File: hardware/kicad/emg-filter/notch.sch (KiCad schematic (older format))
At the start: 9 parts, among them U1 LM4565

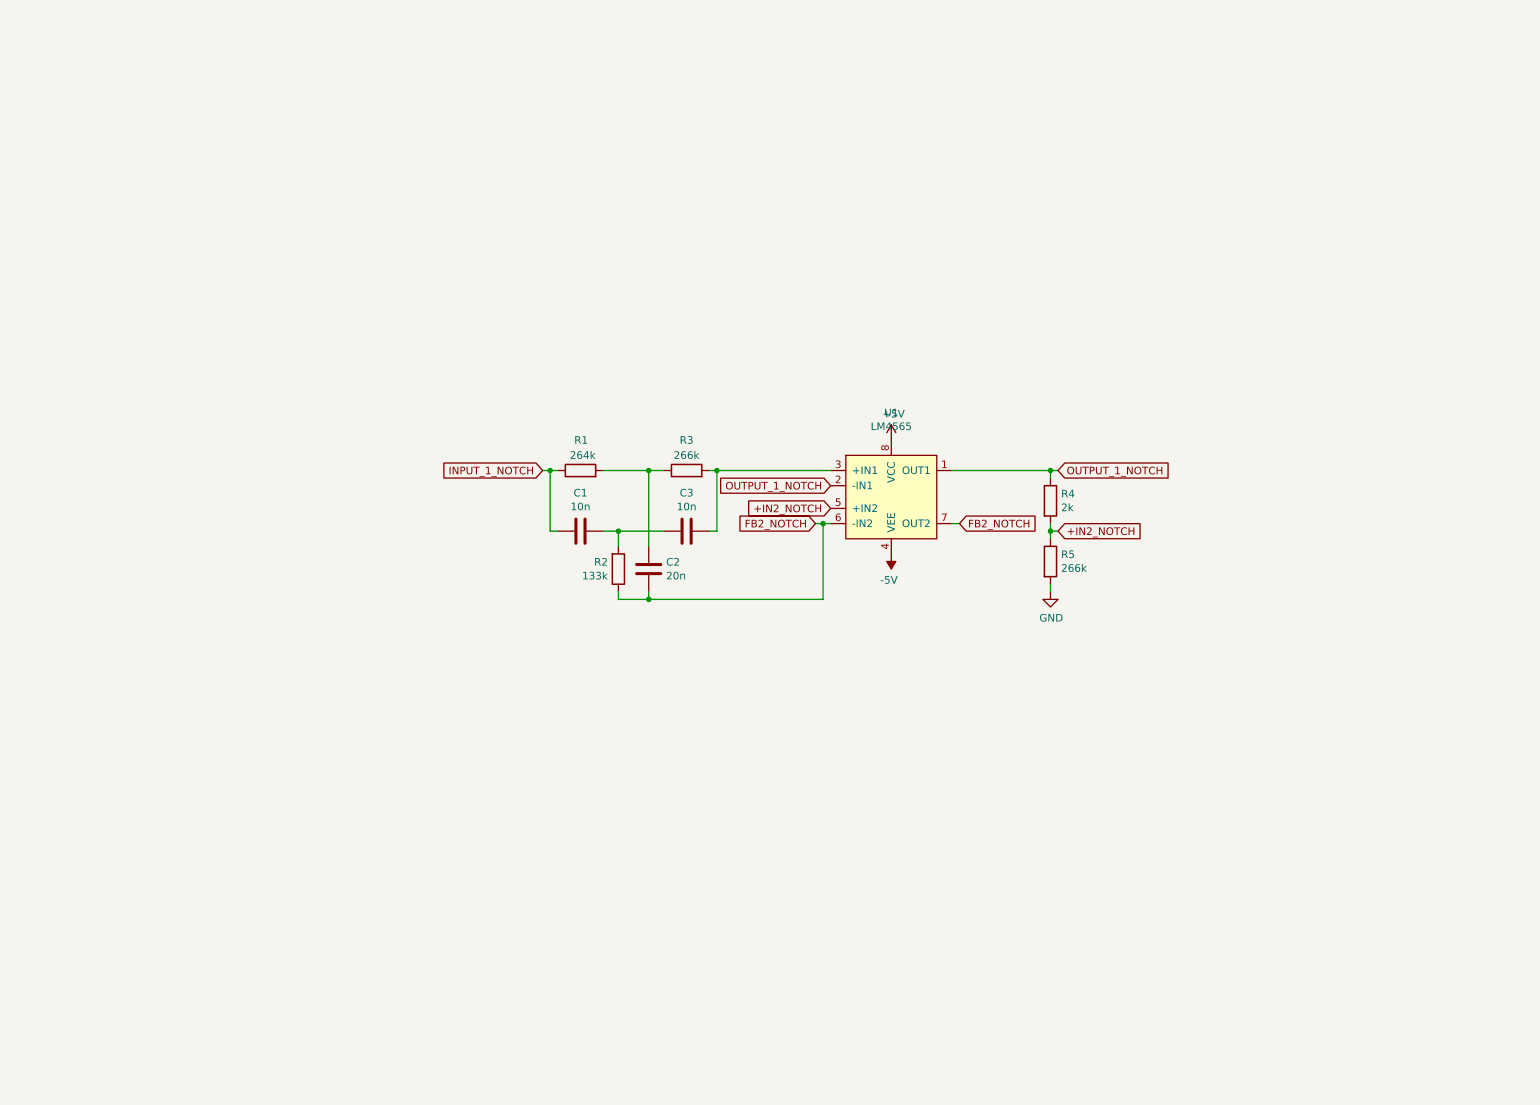
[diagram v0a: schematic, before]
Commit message: notch x16
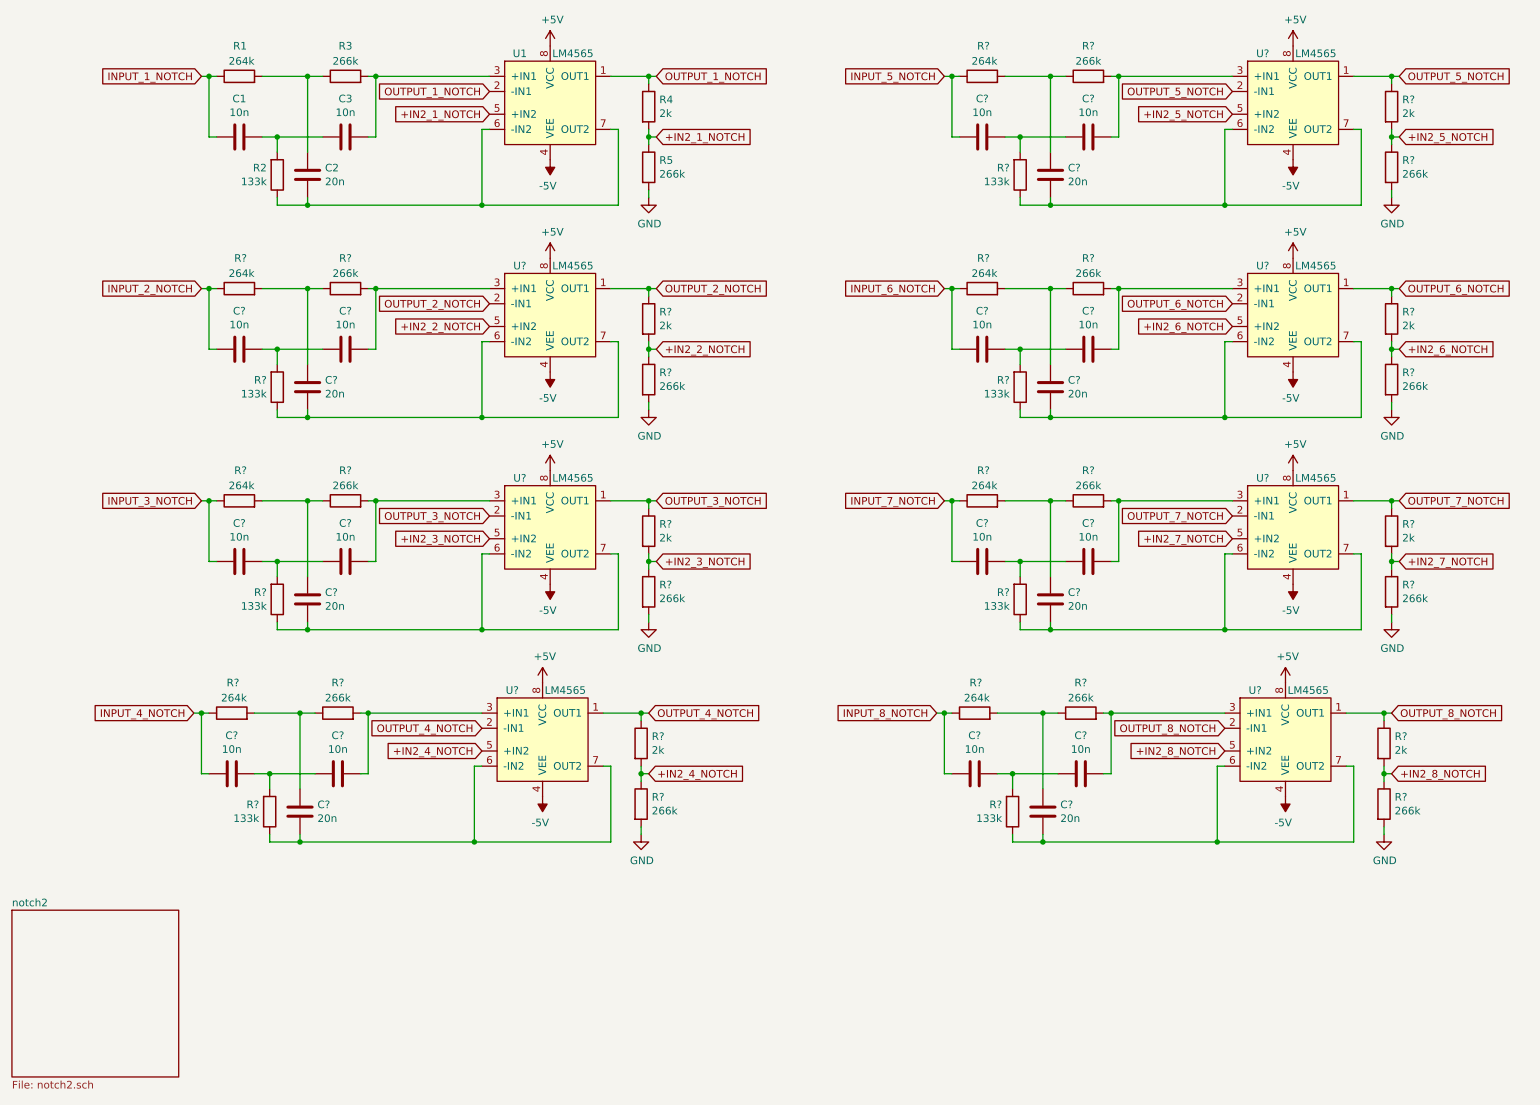
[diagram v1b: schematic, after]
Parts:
- added C? (x7): 20n, symbol Device:C
- added C? (x14): 10n, symbol Device:C
- added R? (x14): 266k, symbol Device:R
- added R? (x7): 133k, symbol Device:R
- added R? (x7): 2k, symbol Device:R
- added R? (x7): 264k, symbol Device:R
- added U? (x7): LM4565, symbol emg-filter:LM4565
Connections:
- net +5V: now also U?.8 (VCC), U?.8 (VCC), U?.8 (VCC), U?.8 (VCC), U?.8 (VCC), U?.8 (VCC), U?.8 (VCC)
- net -5V: now also U?.4 (VEE), U?.4 (VEE), U?.4 (VEE), U?.4 (VEE), U?.4 (VEE), U?.4 (VEE), U?.4 (VEE)
- net GND: now also R?.2, R?.2, R?.2, R?.2, R?.2, R?.2, R?.2
- net +IN2_NOTCH renamed +IN2_1_NOTCH
- net FB2_NOTCH: no longer names the net of C2.1, R2.1, U1.6 (-IN2), U1.7 (OUT2)
- new net: C?.1, R?.2, U?.3 (+IN1) (x7)
- new net: C?.1, R?.1, U?.6 (-IN2), U?.7 (OUT2) (x7)
- new net: C?.2, R?.1, R?.2 (x7)
- new net: C?.1, C?.2, R?.2 (x7)
- new net +IN2_2_NOTCH: R?.1, R?.2, U?.5 (+IN2)
- new net +IN2_3_NOTCH: R?.1, R?.2, U?.5 (+IN2)
- new net +IN2_4_NOTCH: R?.1, R?.2, U?.5 (+IN2)
- new net +IN2_5_NOTCH: R?.1, R?.2, U?.5 (+IN2)
- new net +IN2_6_NOTCH: R?.1, R?.2, U?.5 (+IN2)
- new net +IN2_7_NOTCH: R?.1, R?.2, U?.5 (+IN2)
- new net +IN2_8_NOTCH: R?.1, R?.2, U?.5 (+IN2)
- new net INPUT_2_NOTCH: C?.2, R?.1
- new net INPUT_3_NOTCH: C?.2, R?.1
- new net INPUT_4_NOTCH: C?.2, R?.1
- new net INPUT_5_NOTCH: C?.2, R?.1
- new net INPUT_6_NOTCH: C?.2, R?.1
- new net INPUT_7_NOTCH: C?.2, R?.1
- new net INPUT_8_NOTCH: C?.2, R?.1
- new net OUTPUT_2_NOTCH: R?.1, U?.1 (OUT1), U?.2 (-IN1)
- new net OUTPUT_3_NOTCH: R?.1, U?.1 (OUT1), U?.2 (-IN1)
- new net OUTPUT_4_NOTCH: R?.1, U?.1 (OUT1), U?.2 (-IN1)
- new net OUTPUT_5_NOTCH: R?.1, U?.1 (OUT1), U?.2 (-IN1)
- new net OUTPUT_6_NOTCH: R?.1, U?.1 (OUT1), U?.2 (-IN1)
- new net OUTPUT_7_NOTCH: R?.1, U?.1 (OUT1), U?.2 (-IN1)
- new net OUTPUT_8_NOTCH: R?.1, U?.1 (OUT1), U?.2 (-IN1)
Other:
- moved on the sheet: C1, C2, C3, R1, R2, R3, R4, R5, U1
